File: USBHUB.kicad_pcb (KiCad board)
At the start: 6 copper layers, 92 x 92 mm, 249 parts, among them J1 USB_C_Receptacle, J2 R-RJ45R08P-C000, J3 Screw_Terminal_01x02, Q1 SI3421DV, Q2 SI3421DV, T1 G24P02S, U1 CYPD3177_24x, U10 USB_3_Type_A_Molex_484080003, U11 CYUSB3304-68LTXx, U12 TPS20xxC, U13 TPS20xxC, U14 TPS20xxC, U15 RTL8153-VB-CG, U2 TPS54331, U3 TLV75733PDBV, U4 TPS56637RPAR, U5 TVS2200DRVx, U6 PI3USB302-Ax, U7 TUSB522Px, U8 USB_3_Type_A_Molex_484080003, U9 USB_3_Type_A_Molex_484080003, Y1 26MHz, Y2 25MHz 18pF

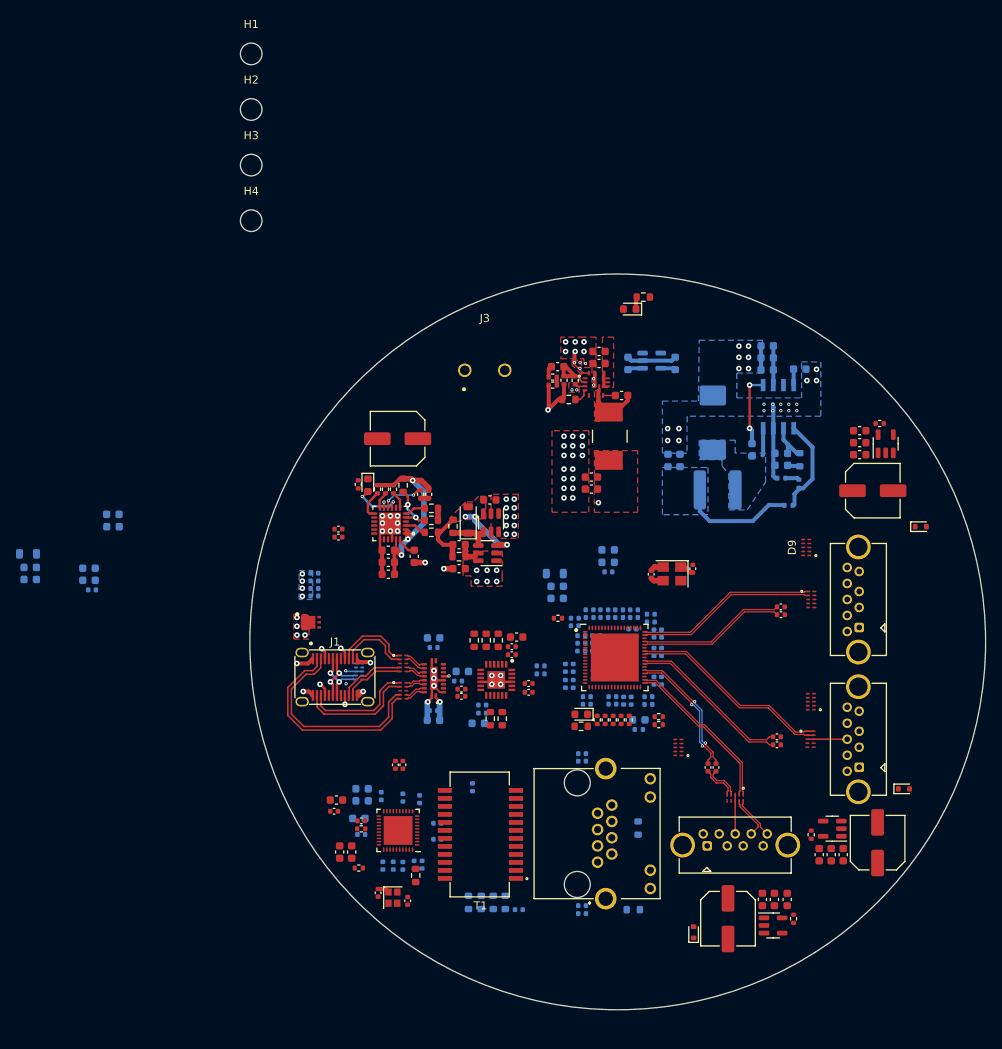
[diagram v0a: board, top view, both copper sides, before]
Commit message: working on pcb
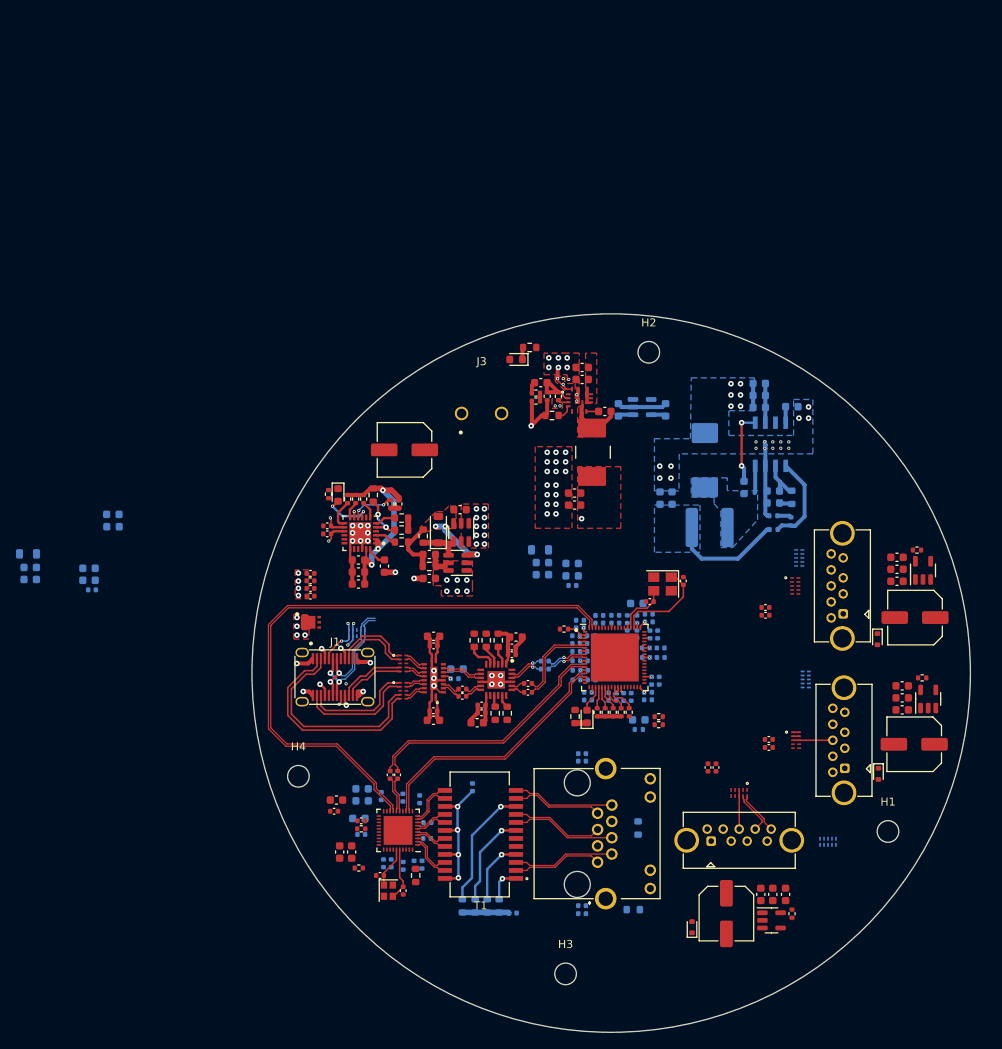
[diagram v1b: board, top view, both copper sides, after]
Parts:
- C26, C27, C28, C29, C35, C36, C37, C38, C40, C41, C42: moved to F.Cu
- D11, D13, D9: moved to B.Cu
- moved H1 125.6 mm to (152.8, 157.3)
- moved H3 108.5 mm to (112.5, 175.1)
- moved H4 69.7 mm to (79.1, 150.4)
- moved H2 58.2 mm to (122.9, 97.4)
- moved R39 24.0 mm to (157.1, 138.1), turned to 0 degrees
- moved C118 23.5 mm to (154.6, 139.1), turned to 0 degrees
- moved D11 22.1 mm to (145.3, 158.6), turned to 180 degrees
- moved C121 21.5 mm to (154.6, 140.6), turned to 0 degrees
- moved U13 20.2 mm to (157.8, 140.7), turned to 90 degrees
- moved C120 19.5 mm to (154.6, 142.1), turned to 0 degrees
- moved C115 16.7 mm to (156.2, 130.6), turned to 180 degrees
- moved C114 16.5 mm to (153.9, 123.0)
- moved C116 16.5 mm to (153.9, 124.5)
- moved C117 16.5 mm to (153.9, 126.0)
- moved R38 16.5 mm to (156.4, 122.1)
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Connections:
- U11 pad 14: HUB1_DS4_RXN -> HUB1_DS4_RXP
- U11 pad 15: HUB1_DS4_RXP -> HUB1_DS4_RXN
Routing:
- net HUB1_DS4_DP: track 0.00 -> 76.6 mm
- net HUB1_DS4_DN: track 0.00 -> 75.6 mm
- net HUB1_DS4_RXP: track 0.00 -> 32.1 mm
- net HUB1_DS4_RXN: track 0.00 -> 31.6 mm
- net /04 Hub Controller/HUB1_DS4_1_TXP: track 0.00 -> 31.4 mm
- net /04 Hub Controller/HUB1_DS4_1_TXN: track 0.00 -> 30.9 mm
- net USB_UFP_CC2: track 0.00 -> 29.7 mm, vias 0 -> 4
- net HUB1_DS2_RXP: track 25.4 -> 0.77 mm
- net HUB1_DS2_RXN: track 25.4 -> 0.77 mm
- net HUB1_DS1_RXP: track 22.6 -> 0.00 mm
- net HUB1_DS1_RXN: track 22.6 -> 0.00 mm
- net HUB1_DS3_RXN: track 26.0 -> 5.46 mm
- net /04 Hub Controller/HUB1_DS2_1_TXN: track 20.3 -> 0.00 mm
- net /04 Hub Controller/HUB1_DS2_1_TXP: track 20.3 -> 0.00 mm
- net HUB1_DS3_RXP: track 25.6 -> 5.46 mm
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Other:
- board size 92 x 92 mm -> 89.8 x 89.8 mm
